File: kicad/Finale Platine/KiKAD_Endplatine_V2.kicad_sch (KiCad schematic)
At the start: 61 parts, among them J1 Conn_02x08_Odd_Even, J4 Conn_01x03_Pin, Q1 Q_NPN_ECB, Q2 Q_NPN_ECB, Q3/+1 Q_NPN_ECB, U1 NE555P, U2 TL074

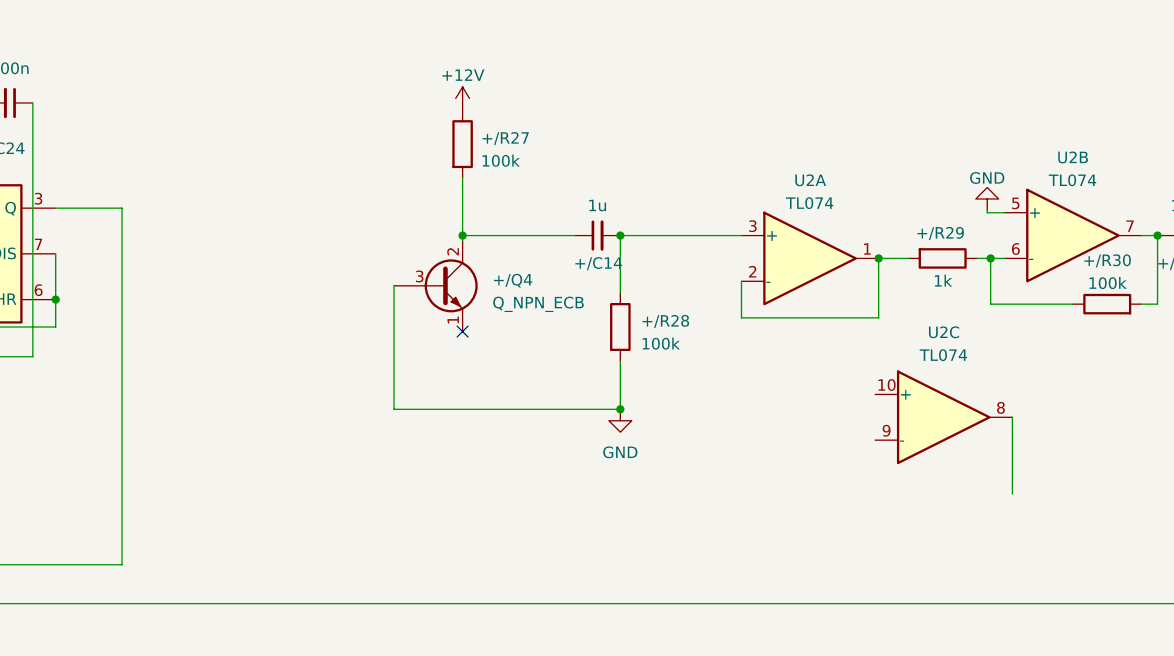
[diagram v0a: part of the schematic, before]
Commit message: noch endgültigere finalplatine
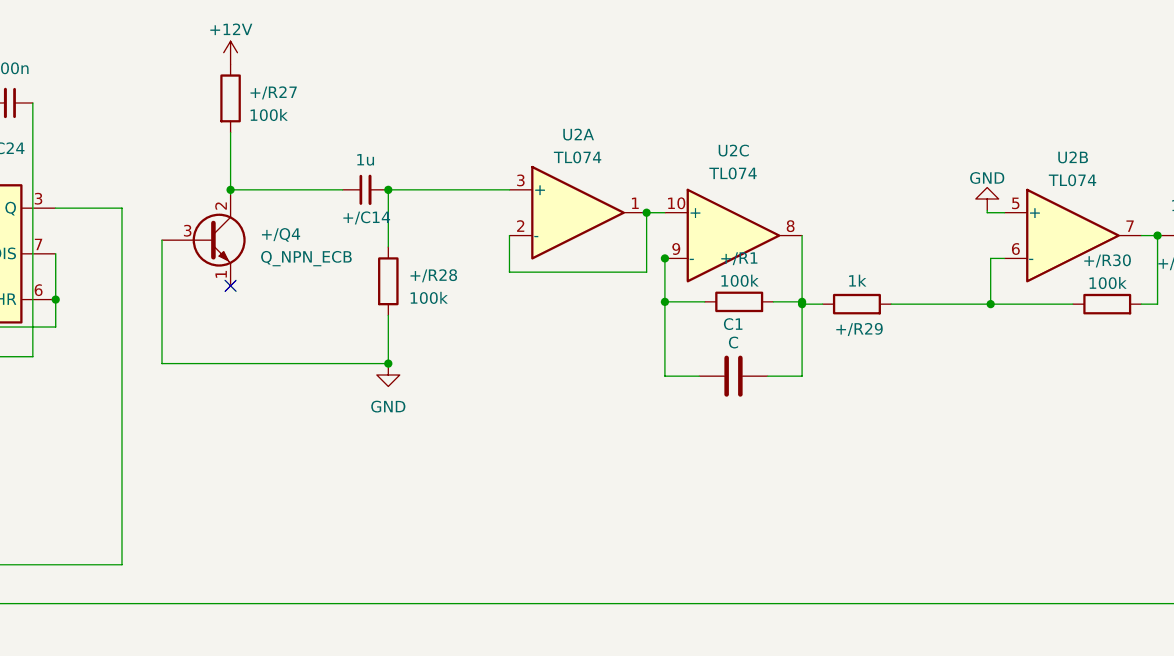
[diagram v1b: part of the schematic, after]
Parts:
- added +/R1: 100k, Resistor_SMD:R_1206_3216Metric_Pad1.30x1.75mm_HandSolder, symbol Device:R
- added C1: C, symbol Device:C
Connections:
- net at +/R30.1, U2.6 (-): now also +/R29.2; no longer +/R29.1
- net at U2.1, U2.2 (-): now also U2.10 (+); no longer +/R29.2
- net at U2.8: now also +/R29.1, +/R1.2, C1.2
- net at U2.9 (-): now also +/R1.1, C1.1
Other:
- moved on the sheet: +/C14, +/Q4, +/R27, +/R28, +/R29, U2A, U2C
